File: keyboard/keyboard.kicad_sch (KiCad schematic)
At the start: 9 parts, among them J1 Conn_01x14

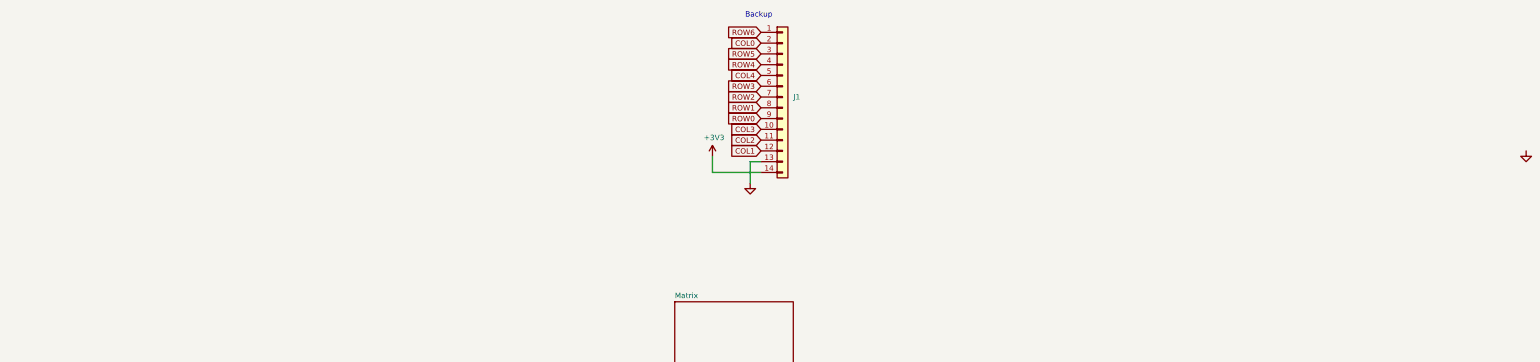
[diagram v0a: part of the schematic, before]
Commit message: keyboard done
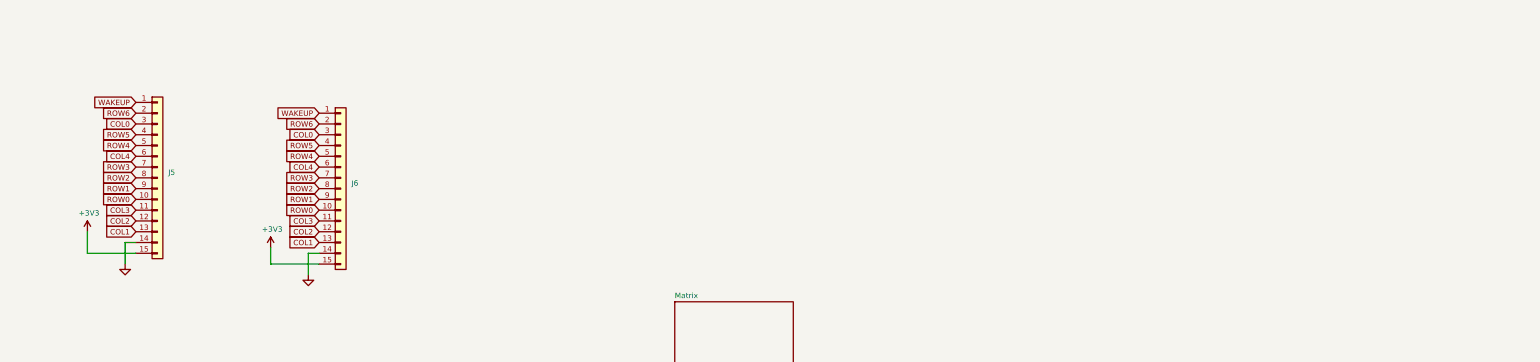
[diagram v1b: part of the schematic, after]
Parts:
- removed J1: Conn_01x14, Connector_PinHeader_2.54mm:PinHeader_1x14_P2.54mm_Vertical, symbol Connector_Generic:Conn_01x14
- added J5: Conn_01x15, Connector_PinHeader_2.54mm:PinHeader_1x15_P2.54mm_Vertical, symbol Connector_Generic:Conn_01x15
- added J6: Conn_01x15, Connector_FFC-FPC:TE_1-84952-5_1x15-1MP_P1.0mm_Horizontal, symbol Connector_Generic:Conn_01x15
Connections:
- net +3V3: now also J5.15 (Pin_15), J6.15 (Pin_15)
- net COL0: now also J5.3 (Pin_3), J6.3 (Pin_3)
- net COL1: now also J5.13 (Pin_13), J6.13 (Pin_13)
- net COL2: now also J5.12 (Pin_12), J6.12 (Pin_12)
- net COL3: now also J5.11 (Pin_11), J6.11 (Pin_11)
- net COL4: now also J5.6 (Pin_6), J6.6 (Pin_6)
- net GND: now also J5.14 (Pin_14), J6.14 (Pin_14)
- net ROW0: now also J5.10 (Pin_10), J6.10 (Pin_10)
- net ROW1: now also J5.9 (Pin_9), J6.9 (Pin_9)
- net ROW2: now also J5.8 (Pin_8), J6.8 (Pin_8)
- net ROW3: now also J5.7 (Pin_7), J6.7 (Pin_7)
- net ROW4: now also J5.5 (Pin_5), J6.5 (Pin_5)
- net ROW5: now also J5.4 (Pin_4), J6.4 (Pin_4)
- net ROW6: now also J5.2 (Pin_2), J6.2 (Pin_2)
- new net WAKEUP: J5.1 (Pin_1), J6.1 (Pin_1)
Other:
- note removed: "Backup"
